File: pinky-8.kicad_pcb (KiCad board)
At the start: 2 copper layers, 91.4 x 68.6 mm, 21 parts, among them P1 USB_B, P2 PERIPHERAL A, P3 PERIPHERAL B, P4 2x3 HEADER, U1 W65C02S, U2 74AC00, U3 AS6C62256, U4 DS1813, U5 GLS29EE010, U6 W65C22S, X1 MXO45

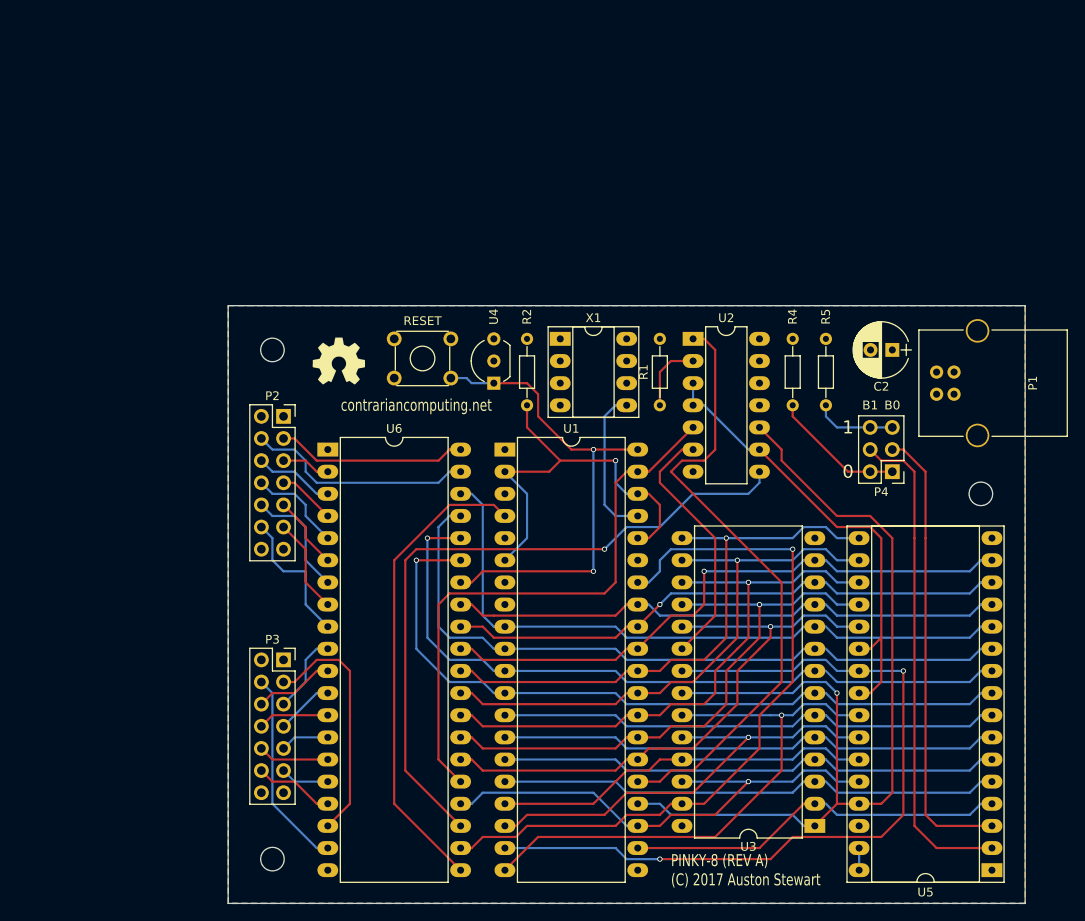
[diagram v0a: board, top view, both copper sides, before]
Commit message: Updating to Rev B spec.
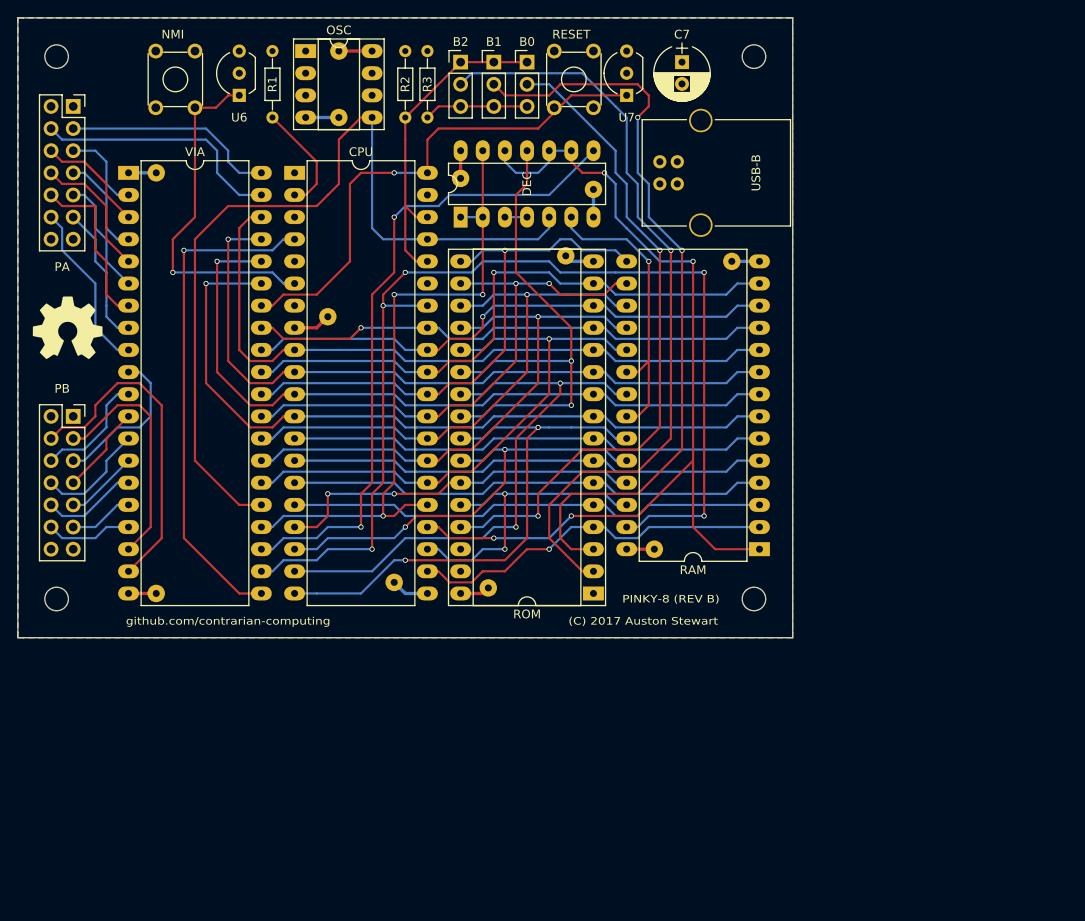
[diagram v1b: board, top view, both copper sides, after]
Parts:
- removed C2: 100uF, Capacitors_THT:CP_Radial_D6.3mm_P2.50mm
- removed the G*** at (118.1, 66.0)
- removed R4, R5: 3.3K, Resistors_THT:R_Axial_DIN0204_L3.6mm_D1.6mm_P7.62mm_Horizontal
- removed the REF** at (110.5, 123.2)
- removed the REF** at (191.8, 81.3)
- removed the REF** at (110.5, 64.8)
- removed U1: W65C02S, Housings_DIP:DIP-40_W15.24mm_LongPads
- removed U2: 74AC00, Housings_DIP:DIP-14_W7.62mm_LongPads
- removed U3: AS6C62256, Housings_DIP:DIP-28_W15.24mm_LongPads
- removed U4: DS1813, TO_SOT_Packages_THT:TO-92_Inline_Wide
- removed U5: GLS29EE010, Housings_DIP:DIP-32_W15.24mm_Socket_LongPads
- removed X1: MXO45, Housings_DIP:DIP-8_W7.62mm_Socket_LongPads
- added B0: CONN_01X03, Pin_Headers:Pin_Header_Straight_1x03_Pitch2.54mm, F.Cu at (139.7, 31.8)
- added B1: CONN_01X03, Pin_Headers:Pin_Header_Straight_1x03_Pitch2.54mm, F.Cu at (135.9, 31.8)
- added B2: CONN_01X03, Pin_Headers:Pin_Header_Straight_1x03_Pitch2.54mm, F.Cu at (132.1, 31.8)
- added C7: 100uF, Capacitors_THT:CP_Radial_D6.3mm_P2.50mm, F.Cu at (157.5, 31.8)
- added CPU: W65C02S, Housings_DIP:DIP-40_W15.24mm_LongPads, F.Cu at (113.0, 44.5)
- added DEC: 74AC00, Housings_DIP:DIP-14_W7.62mm_LongPads, F.Cu at (132.1, 49.5)
- added G***: OSHW-logo_silkscreen-front_8mm, OSHW-logo:OSHW-logo_silkscreen-front_8mm, F.Cu at (87.0, 62.2)
- added NMI: SW_Push_Dual, Buttons_Switches_THT:SW_TH_Tactile_Omron_B3F-10xx, F.Cu at (101.6, 30.5)
- added OSC: MXO45, Housings_DIP:DIP-8_W7.62mm_Socket_LongPads, F.Cu at (114.3, 30.5)
- added P10: CONN_01X01, Wire_Pads:SolderWirePad_single_0-8mmDrill, F.Cu at (135.3, 92.1)
- added P11: CONN_01X01, Wire_Pads:SolderWirePad_single_0-8mmDrill, F.Cu at (154.3, 87.6)
- added P13: CONN_01X01, Wire_Pads:SolderWirePad_single_0-8mmDrill, F.Cu at (124.5, 91.4)
- added P14: CONN_01X01, Wire_Pads:SolderWirePad_single_0-8mmDrill, F.Cu at (144.1, 54.0)
- added P15: CONN_01X01, Wire_Pads:SolderWirePad_single_0-8mmDrill, F.Cu at (116.8, 61.0)
- added P17: CONN_01X01, Wire_Pads:SolderWirePad_single_0-8mmDrill, F.Cu at (97.2, 44.5)
- added P5: CONN_01X01, Wire_Pads:SolderWirePad_single_0-8mmDrill, F.Cu at (147.3, 46.4)
- added P6: CONN_01X01, Wire_Pads:SolderWirePad_single_0-8mmDrill, F.Cu at (163.2, 54.6)
- added PA: PERIPHERAL A, Socket_Strips:Socket_Strip_Straight_2x07_Pitch2.54mm, F.Cu at (87.6, 36.8)
- added PB: PERIPHERAL B, Socket_Strips:Socket_Strip_Straight_2x07_Pitch2.54mm, F.Cu at (87.6, 72.4)
- added R3: 3.3K, Resistors_THT:R_Axial_DIN0204_L3.6mm_D1.6mm_P7.62mm_Horizontal, F.Cu at (128.3, 38.1)
- added RAM: AS6C62256, Housings_DIP:DIP-28_W15.24mm_LongPads, F.Cu at (166.4, 87.6)
- added REF**: MountingHole_2.7mm_M2.5, Mounting_Holes:MountingHole_2.7mm_M2.5, F.Cu at (165.7, 31.1)
- added REF**: MountingHole_2.7mm_M2.5, Mounting_Holes:MountingHole_2.7mm_M2.5, F.Cu at (165.7, 93.3)
- added REF**: MountingHole_2.7mm_M2.5, Mounting_Holes:MountingHole_2.7mm_M2.5, F.Cu at (85.7, 93.3)
- added REF**: MountingHole_2.7mm_M2.5, Mounting_Holes:MountingHole_2.7mm_M2.5, F.Cu at (85.7, 31.1)
- added ROM: GLS29EE010, Housings_DIP:DIP-32_W15.24mm_Socket_LongPads, F.Cu at (147.3, 92.7)
- added U7: DS1813, TO_SOT_Packages_THT:TO-92_Inline_Wide, F.Cu at (151.1, 35.6)
- added USB-B: USB_B, Connectors:USB_B, F.Cu at (154.9, 43.2)
- added VIA: W65C22S, Housings_DIP:DIP-40_W15.24mm_LongPads, F.Cu at (94.0, 44.5)
- P1: value USB_B -> CONN_01X01; footprint Connectors:USB_B -> Wire_Pads:SolderWirePad_single_0-8mmDrill
- P2: value PERIPHERAL A -> CONN_01X01; footprint Socket_Strips:Socket_Strip_Straight_2x07_Pitch2.54mm -> Wire_Pads:SolderWirePad_single_0-8mmDrill
- P3: value PERIPHERAL B -> CONN_01X01; footprint Socket_Strips:Socket_Strip_Straight_2x07_Pitch2.54mm -> Wire_Pads:SolderWirePad_single_0-8mmDrill
- P4: value 2x3 HEADER -> CONN_01X01; footprint Pin_Headers:Pin_Header_Straight_2x03_Pitch2.54mm -> Wire_Pads:SolderWirePad_single_0-8mmDrill
- U6: value W65C22S -> DS1813; footprint Housings_DIP:DIP-40_W15.24mm_LongPads -> TO_SOT_Packages_THT:TO-92_Inline_Wide
- moved P1 77.8 mm to (118.1, 30.5)
- moved P4 75.4 mm to (118.1, 38.1), turned to 0 degrees
- moved R1 60.2 mm to (110.5, 30.5), turned to 270 degrees
- moved U6 41.9 mm to (106.7, 35.6), turned to 90 degrees
- moved RESET 40.2 mm to (147.3, 30.5), turned to 270 degrees
- moved P2 34.0 mm to (132.1, 45.1)
- moved R2 29.0 mm to (125.7, 38.1), turned to 90 degrees
- moved P3 16.5 mm to (97.2, 92.7)
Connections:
- P4 pad 1: Net-(P4-Pad1) -> GND
- R1 pad 1: Net-(R1-Pad1) -> VCC
- R1 pad 2: VCC -> Net-(R1-Pad2)
- R2 pad 1: VCC -> /PLUP
- R2 pad 2: Net-(R2-Pad2) -> VCC
- RESET pad 4: /RST -> /RST#
- U6 pad 1: GND -> /NMI#
- U6 pad 2: /PA0 -> VCC
- U6 pad 3: /PA1 -> GND
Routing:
- net /RW#: track 0.00 -> 124.9 mm, vias 0 -> 5
- net /RB2: track 0.00 -> 88.2 mm, vias 0 -> 1
- net /RW: track 83.6 -> 0.00 mm, vias 1 -> 0
- net /CLK: track 17.6 -> 99.5 mm
- net /VIASEL: track 78.7 -> 0.00 mm, vias 2 -> 0
- net /VIASEL#: track 0.00 -> 75.6 mm, vias 0 -> 2
- net /PHI2: track 65.7 -> 0.00 mm
- net /RST#: track 0.00 -> 59.7 mm, vias 0 -> 1
- net /ROMSEL#: track 0.00 -> 58.8 mm, vias 0 -> 2
- net /IRQ#: track 0.00 -> 57.8 mm, vias 0 -> 1
- net /RST: track 56.1 -> 0.00 mm, vias 3 -> 0
- net /IRQ: track 54.6 -> 0.00 mm
- net /ROMSEL: track 53.1 -> 0.00 mm
- net Net-(R2-Pad2): track 47.7 -> 0.00 mm, vias 1 -> 0
- net /NMI#: track 0.00 -> 40.1 mm, vias 0 -> 1
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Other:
- board size 91.4 x 68.6 mm -> 88.9 x 71.1 mm
- net class Power added: clearance 0.25, trace_width 0.38, via_dia 0.4, via_drill 0.3
- rule pad_to_mask_clearance: 0.2 -> 0
- rule trace_min: 0.1524 -> 0.2
- board text added: "(C) 2017 Auston Stewart"
- board text added: "PINKY-8 (REV B)"
- board text added: "github.com/contrarian-computing"
- board text removed: "0"
- board text removed: "1"
- board text removed: "B0"
- board text removed: "B1"
- board text removed: "PINKY-8 (REV A) (C) 2017 Auston Stewart"
- board text removed: "contrariancomputing.net"
